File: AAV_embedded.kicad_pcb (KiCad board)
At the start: 4 copper layers, 168.2 x 114.7 mm, 94 parts, among them J1 JTAG_SWD_CONN, J10 DRV_HIGH_C2, J11 DRV_LOW_C2, J12 DRV_HIGH_C3, J13 DRV_LOW_C3, J14 DRV_LOW_C1, J15 Brake/FwRev, J16 5v_in, J17 3.3v_in, J18 12v_in, J2 Raspberry_Pi_4, J21 CAN, J23 5v_rail, J24 3.3v_rail, J25 12v_rail, J26 GND_rail, J27 12v_rail_f, J28 3.3v_rail_f, J29 5v_rail_f, J3 USB_C_Receptacle_USB2.0_14P, J30 GND_rail_f, J32 Conn_02x15_Counter_Clockwise, J34 Conn_02x15_Counter_Clockwise, J5 THR_EN_JMP, J6 Conn_01x07, J7 Conn_01x05, J8 Throttle Connector, J9 DRV_HIGH_C1, SW10 SW_DIP_x02, SW2 IO_EXT_ADDR, SW4 5v_USB_EN, SW5 THR_EN, SW6 ~{RESET_uMOD}, SW7 ~{BOOT_uMOD}, SW8 ~{RESET_BRK}, SW9 ~{RESET_STR}, U1 DAC101C081CIMK, U2 PCA9555D, U3 74AHC1G08, U5 FXMA108, U6 MCP2515-xSO, U7 SN65HVD230, Y1 16MHz

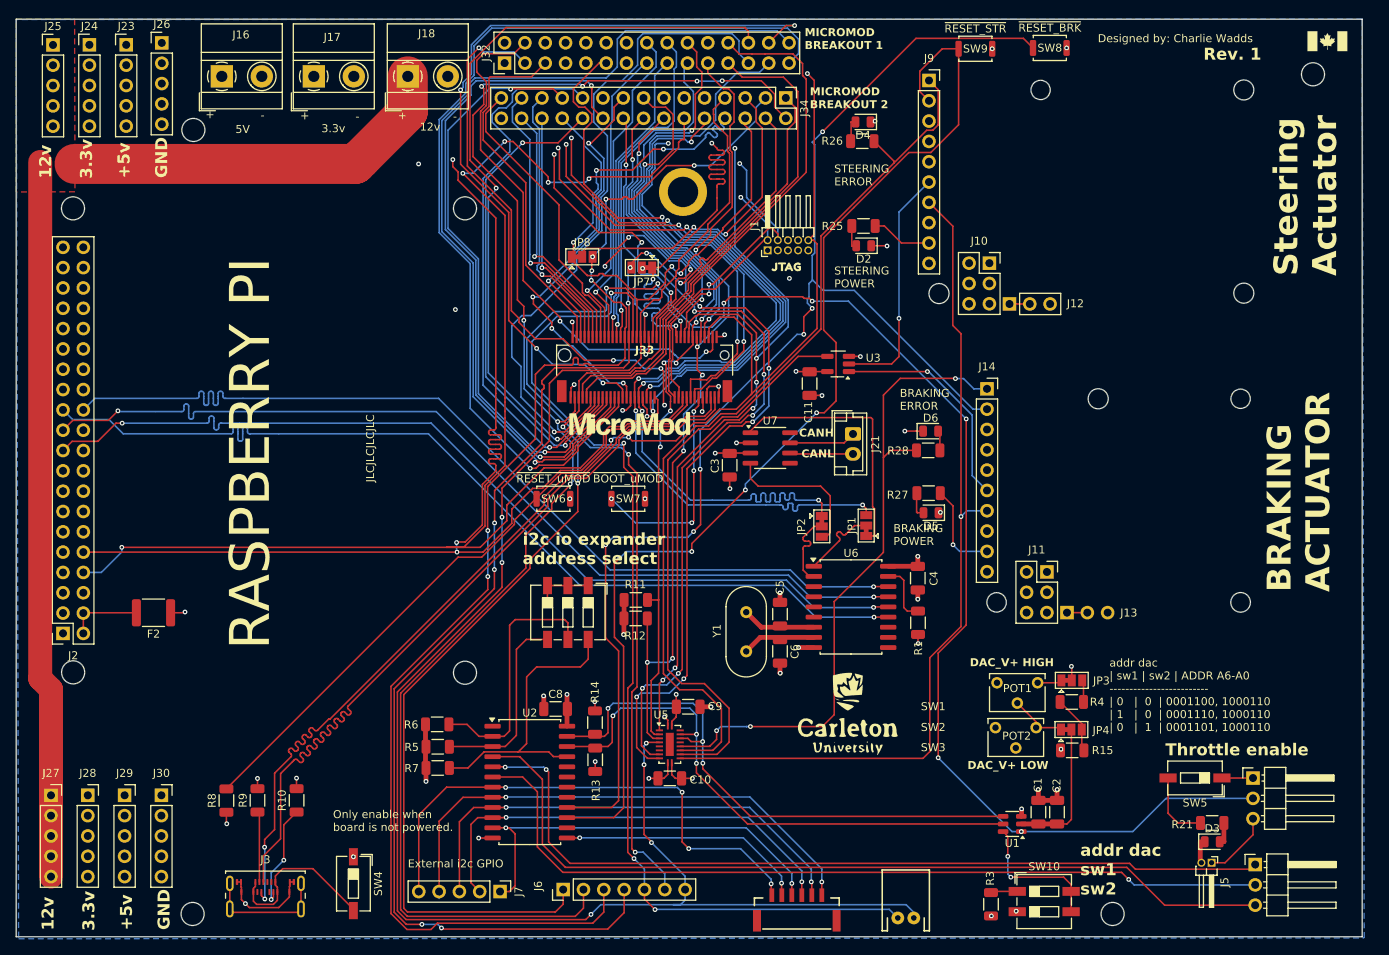
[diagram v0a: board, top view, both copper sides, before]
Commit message: new branch with fixes
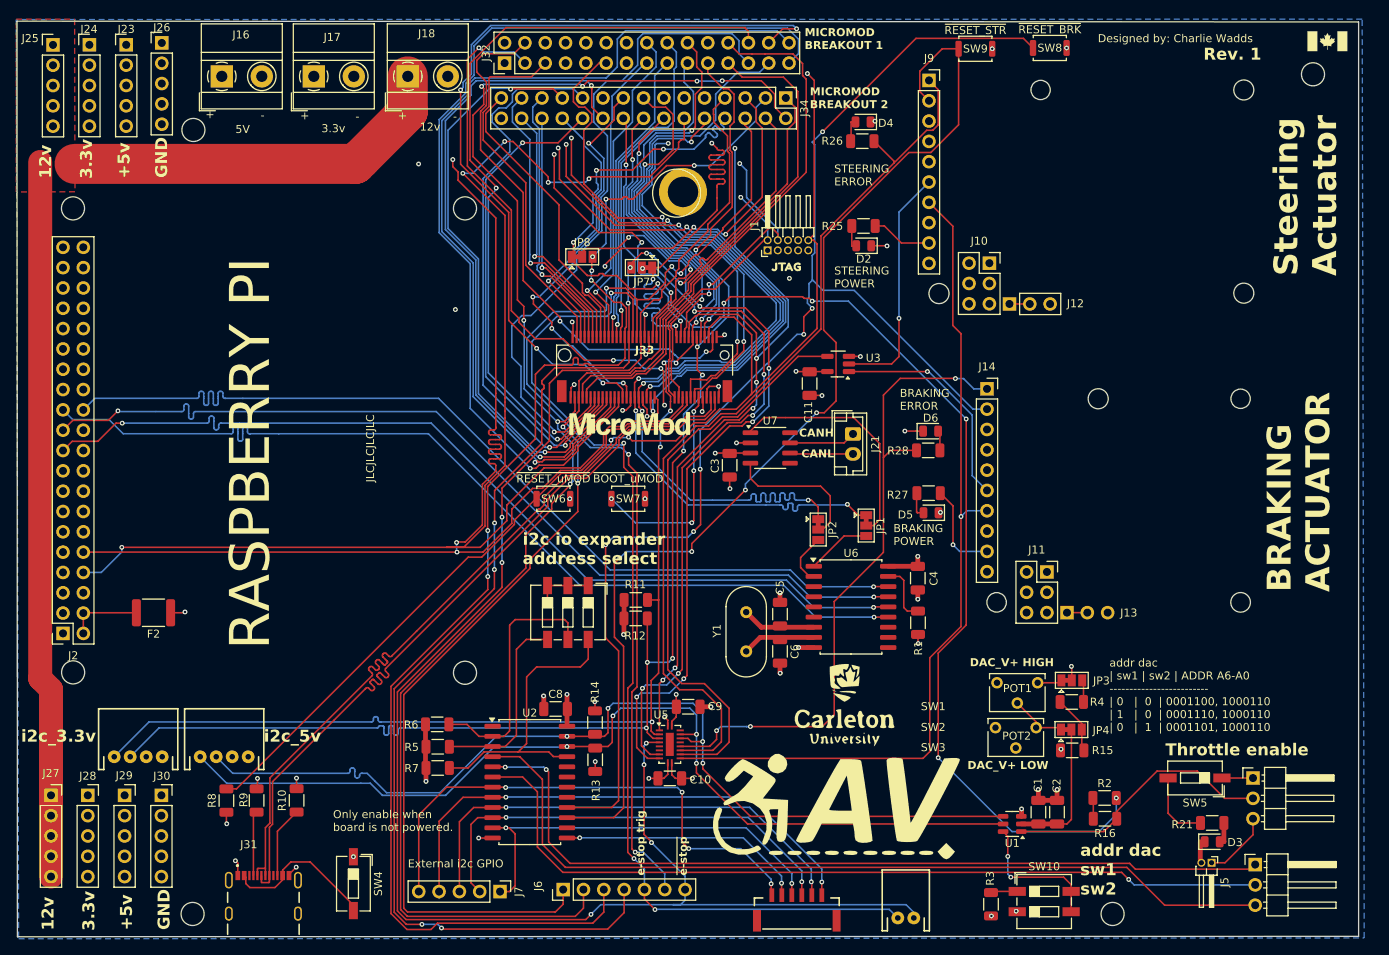
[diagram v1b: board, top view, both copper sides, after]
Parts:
- removed J3: USB_C_Receptacle_USB2.0_14P, Connector_USB:USB_C_Receptacle_Amphenol_124019772112A
- added G***: LOGO, LOGO, F.Cu at (151.2, 141.6)
- added J22: ~, SparkFun-Connectors:JST-4-PTH, F.Cu at (63.2, 135.3)
- added J31: USB4520-03-0-A_REVA, USB4105_GF_A:GCT_USB4105-GF-A, F.Cu at (78.8, 155.0)
- added J4: ~, SparkFun-Connectors:JST-4-PTH, F.Cu at (74.0, 135.3)
- added R16: 10k, Resistor_SMD:R_1206_3216Metric, F.Cu at (184.1, 143.1)
- added R2: 10k, Resistor_SMD:R_1206_3216Metric, F.Cu at (184.0, 140.5)
- R10: value 10k -> 5.1k
- moved G*** 1.17 mm to (151.5, 128.9)
- moved JP2 0.60 mm to (148.2, 107.0)
- moved R9 0.11 mm to (78.0, 140.8)
- turned JP1 to -90 degrees
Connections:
- J8 pad 2: A0 -> DAC_THR
- JP1 pad 1: Net-(JP1-A) -> CAN_TXD
- JP1 pad 2: CAN_TXD_PI -> Net-(JP1-C)
- JP1 pad 3: CAN_TXD -> CAN_TXD_PI
- JP2 pad 2: CAN_RXD_PI -> Net-(JP2-C)
- JP2 pad 3: Net-(JP2-B) -> CAN_RXD_PI
- U1 pad 1: A0 -> DAC_THR
- U7 pad 1: Net-(JP1-A) -> Net-(JP1-C)
- U7 pad 4: Net-(JP2-B) -> Net-(JP2-C)
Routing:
- net SCL_1_L: track 105.9 -> 175.8 mm, vias 6 -> 7
- net SDA _1_L: track 104.3 -> 174.1 mm, vias 6 -> 7
- net SDA_1_H: track 70.9 -> 121.3 mm, vias 3 -> 4
- net SCL_1_H: track 71.0 -> 121.3 mm, vias 3 -> 4
- net DAC_THR: track 0.00 -> 34.0 mm
- net Net-(JP1-A): track 31.9 -> 0.00 mm
- net Net-(JP1-C): track 0.00 -> 29.9 mm
- net Net-(JP2-B): track 18.7 -> 0.00 mm
- net Net-(JP2-C): track 0.00 -> 17.9 mm
- net A0: track 180.9 -> 165.0 mm
- net unconnected-(J3-SHIELD-PadS1): track 15.7 -> 0.00 mm
- net GND: track 70.5 -> 61.7 mm, vias 34 -> 35
- net Net-(J31-CC2): track 13.3 -> 8.93 mm, vias 2 -> 0
- net USB-D+: track 100.9 -> 96.8 mm
- net CAN_RXD_PI: track 10.0 -> 6.47 mm
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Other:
- board size 168.2 x 114.7 mm -> 167.7 x 114.4 mm
- board text added: "e-stop trig"
- board text added: "i2c_3.3v"
- board text added: "i2c_5v"
- board text added: "~{e-stop}"
